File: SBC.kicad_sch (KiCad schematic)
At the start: 0 parts

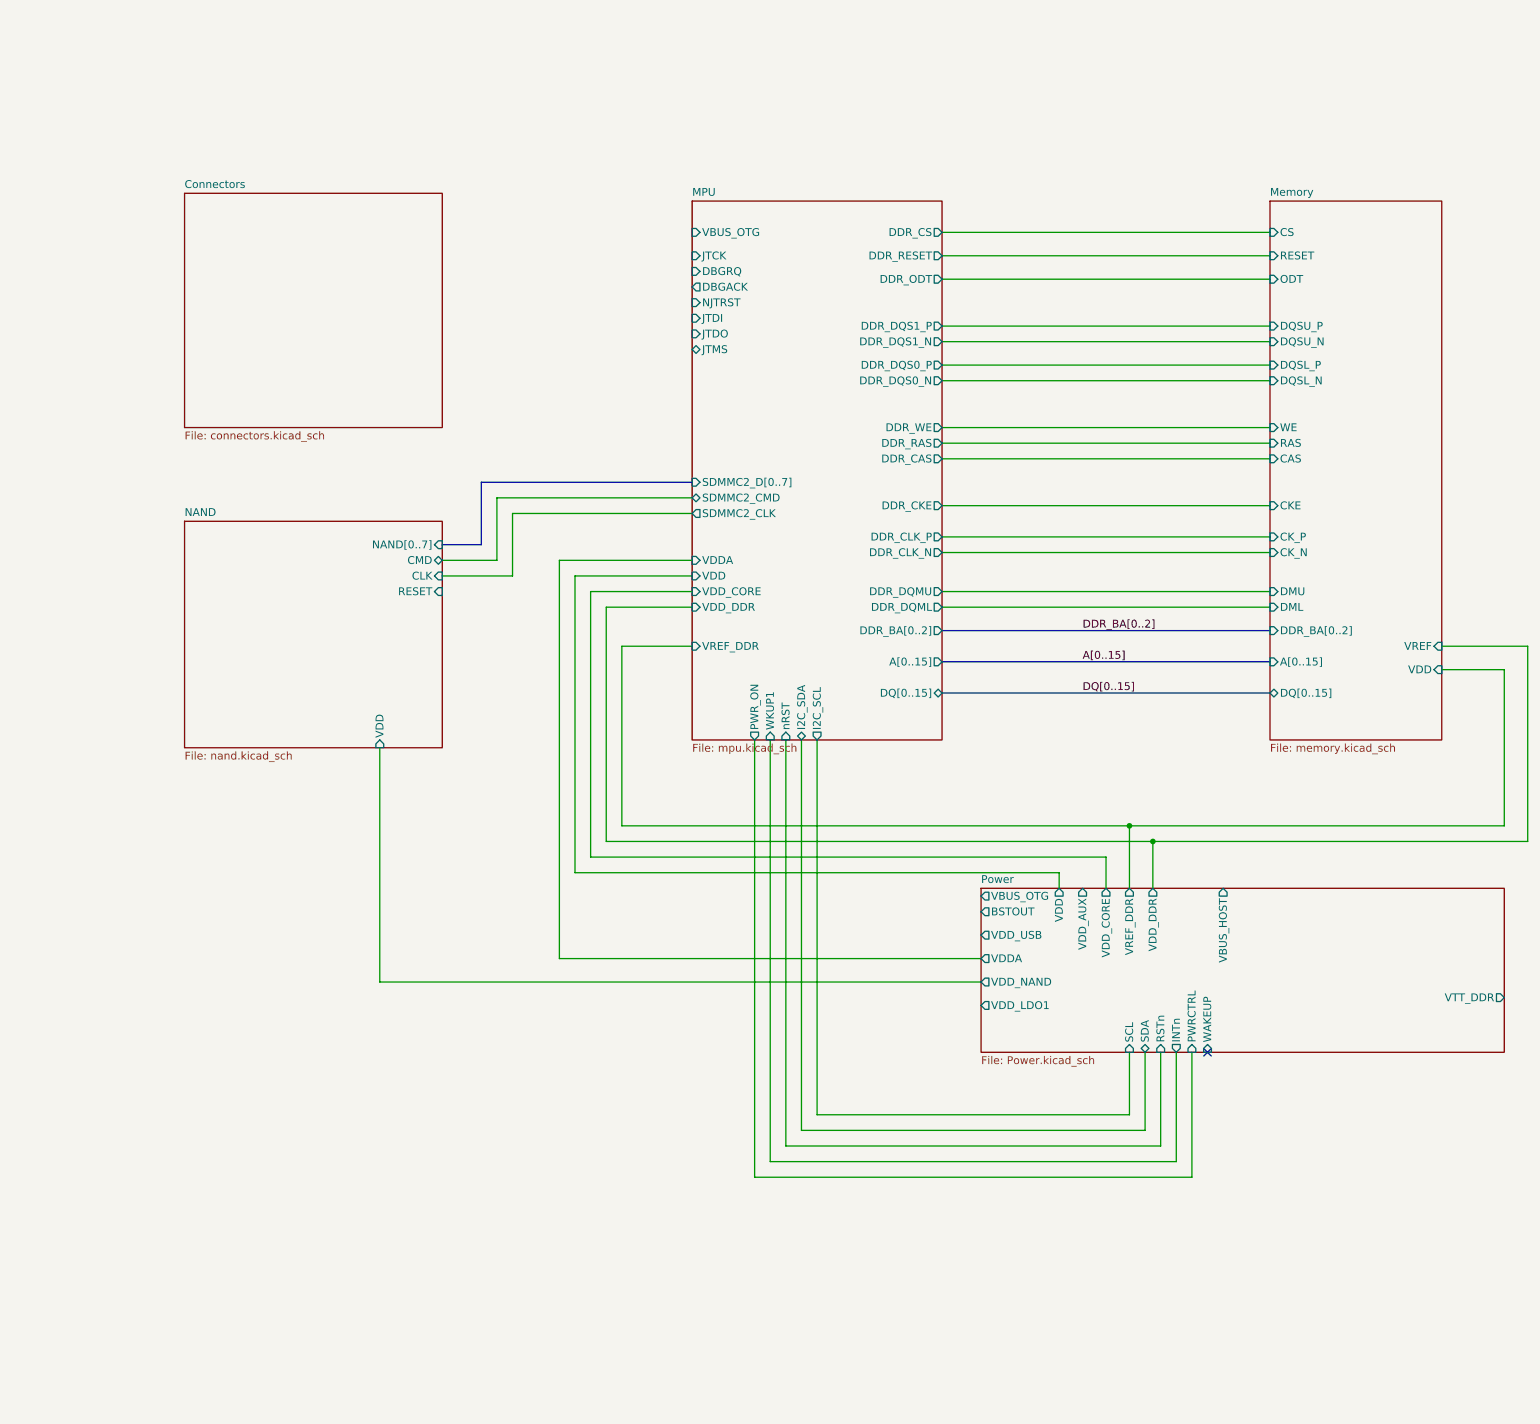
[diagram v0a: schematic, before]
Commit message: Working on Ethernet connections
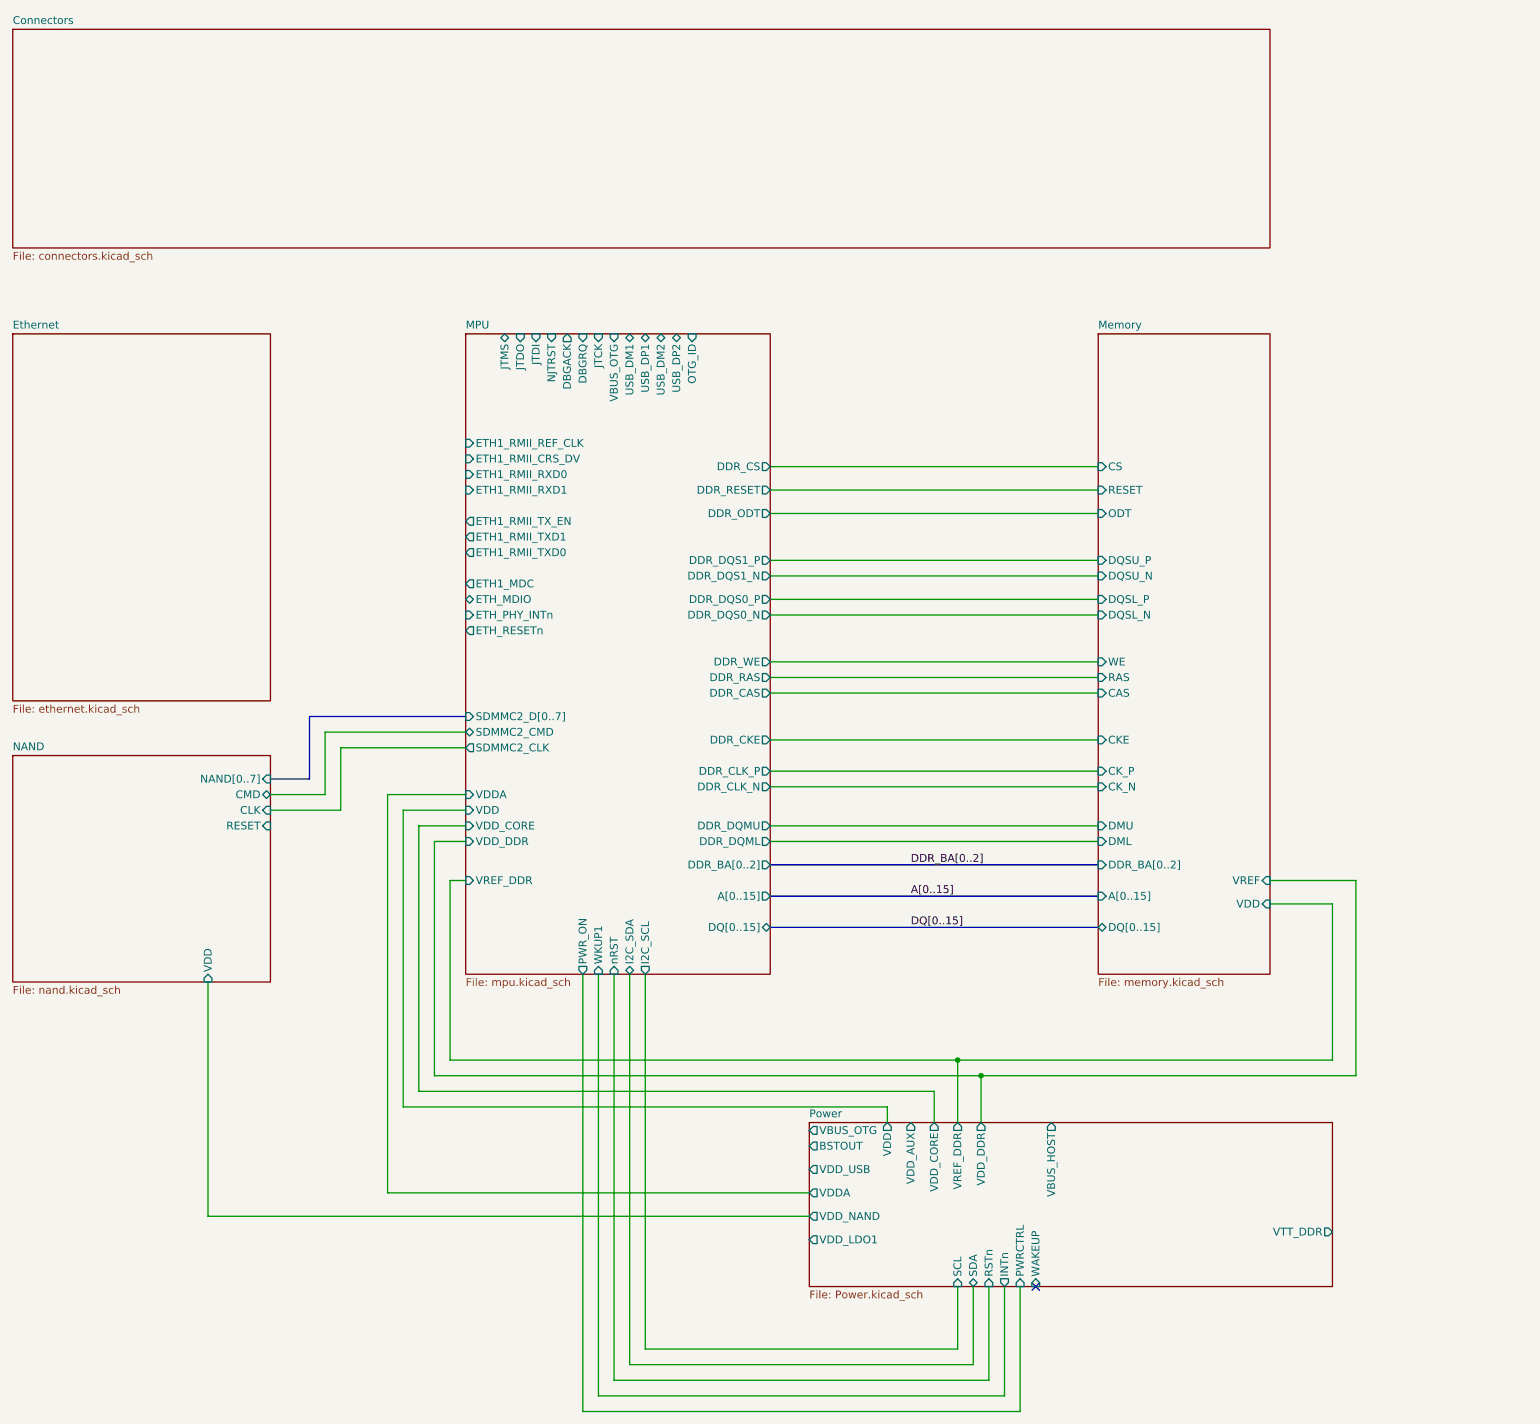
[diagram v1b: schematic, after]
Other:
- added sheet Ethernet (ethernet.kicad_sch)
- sheet MPU ports: added ETH1_MDC, ETH1_RMII_CRS_DV, ETH1_RMII_REF_CLK, ETH1_RMII_RXD0, ETH1_RMII_RXD1, ETH1_RMII_TXD0, ETH1_RMII_TXD1, ETH1_RMII_TX_EN, ETH_MDIO, ETH_PHY_INTn, ETH_RESETn, OTG_ID, USB_DM1, USB_DM2, USB_DP1, USB_DP2; removed none
